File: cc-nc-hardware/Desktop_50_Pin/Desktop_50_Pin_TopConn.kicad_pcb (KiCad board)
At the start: 4 copper layers, 93.7 x 82.6 mm, 112 parts, among them J1 Conn_01x03_Male, J10 Conn_01x03_Male, J11 Conn_01x02_Male, J2 Conn_02x25_Odd_Even, J3 BergFloppy, J4 USB_C_Receptacle, J5 Conn_01x03_Male, J6 SM04B-SRSS-TB(LF)(SN), J7 TERM_BCKF, J8 EPWR, J9 Conn_01x02_Male, Q1 AO3401A, Q2 AO3401A, SW1 SW_MEC_5E, U13 LVT125, U14 LVT125, U15 LVT125, U16 LVT125, U3 AMS1117-2.85, U4 LVT245, U5 LVT245, U6 LVT245, U8 74HC14, U9 LVT245

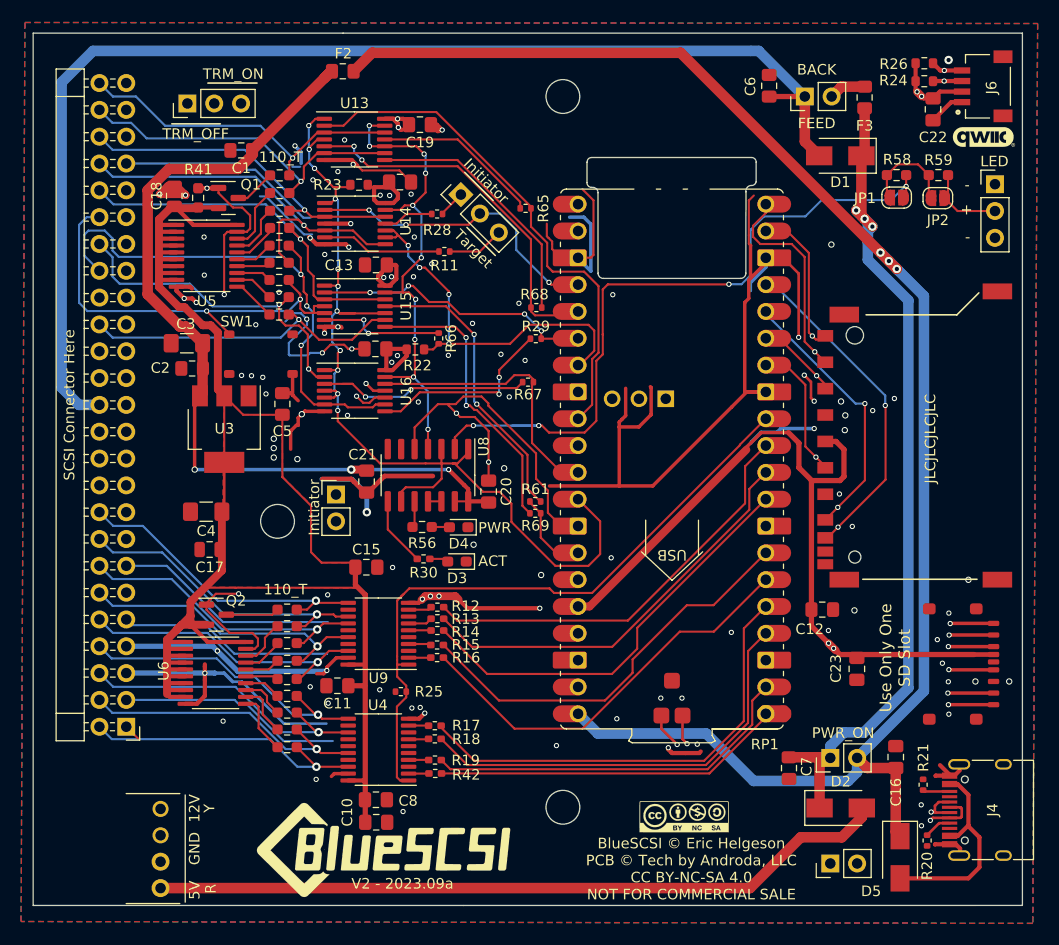
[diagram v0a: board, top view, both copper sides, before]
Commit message: Desktop 2023.10a design
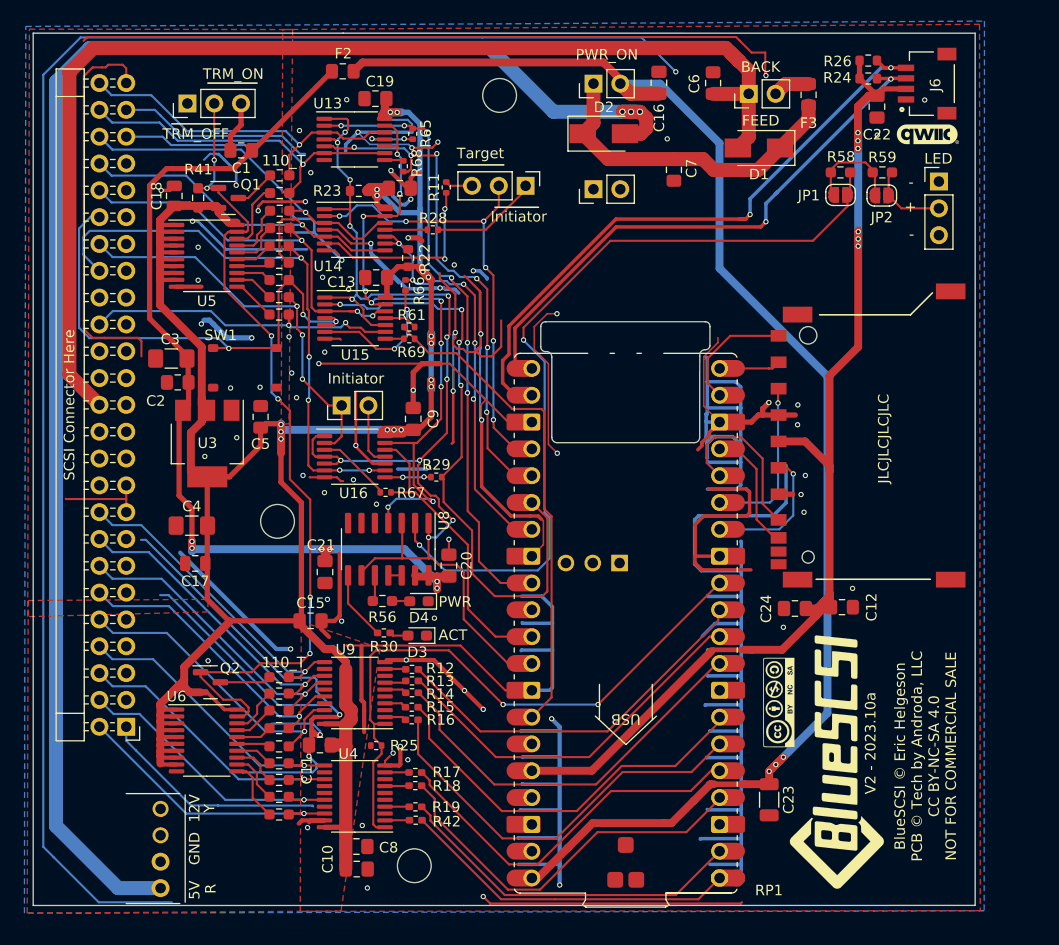
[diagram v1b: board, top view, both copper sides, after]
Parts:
- removed D5: D, Diode_SMD:D_SMA
- removed J4: USB_C_Receptacle, Connector_USB:USB_C_Receptacle_HRO_TYPE-C-31-M-12
- removed R20, R21: 5.1k, Resistor_SMD:R_0402_1005Metric
- removed SD2: MicroSD-TF-06, Library:TF-06_MicroSD
- added C24: 0.1uF, Capacitor_SMD:C_0805_2012Metric_Pad1.18x1.45mm_HandSolder, F.Cu at (172.1, 118.3)
- C23: value 4.7uF -> 20uF; footprint Capacitor_SMD:C_0805_2012Metric_Pad1.18x1.45mm_HandSolder -> Capacitor_SMD:C_1206_3216Metric
- J11: value Conn_01x02_Male -> ACK_En
- moved C16 67.7 mm to (159.3, 68.5)
- moved D2 67.7 mm to (154.0, 73.3)
- moved J8 67.7 mm to (153.1, 68.6)
- moved J9 67.7 mm to (153.1, 78.6)
- moved C7 57.7 mm to (160.7, 76.8)
- moved R61 20.4 mm to (135.6, 91.6)
- moved R69 20.4 mm to (135.6, 92.7)
- moved R68 18.4 mm to (135.1, 76.4), turned to 90 degrees
- moved R67 17.1 mm to (133.4, 107.3)
- moved RP1 16.2 mm to (156.1, 119.8)
- moved R29 16.1 mm to (138.2, 105.8)
- moved H3 15.1 mm to (136.1, 142.6)
- moved C23 14.9 mm to (169.7, 136.4)
- moved G*** 14.0 mm to (170.6, 127.2), turned to 90 degrees
- moved R65 12.8 mm to (135.9, 73.3), turned to 90 degrees
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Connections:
- C23 pad 1: +3V3 -> +5VP
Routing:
- net GND: track 569.8 -> 946.8 mm, vias 100 -> 81
- net Net-(D2-Pad2): track 70.1 -> 151.4 mm, vias 0 -> 3
- net SD_D3_CS: track 58.1 -> 4.21 mm, vias 2 -> 0
- net SD_D1: track 59.6 -> 10.7 mm, vias 3 -> 0
- net +3V3: track 149.2 -> 109.8 mm, vias 4 -> 6
- net SD_D2: track 50.7 -> 11.5 mm, vias 2 -> 0
- net Net-(R61-Pad1): track 7.97 -> 46.5 mm
- net SD_D0_MISO: track 54.6 -> 16.3 mm, vias 3 -> 0
- net Net-(C7-Pad1): track 82.0 -> 45.2 mm, vias 3 -> 0
- net USB_DM: track 35.5 -> 0.00 mm, vias 2 -> 0
- net USB_DP: track 33.0 -> 0.00 mm, vias 2 -> 0
- net oMSG_iBSY: track 25.4 -> 58.0 mm
- net SD_CLK: track 45.1 -> 13.1 mm, vias 2 -> 1
- net SD_CMD_MOSI: track 44.9 -> 16.0 mm, vias 2 -> 1
- net +5F: track 121.4 -> 93.3 mm, vias 3 -> 6
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- removed copper zone on In1.Cu, net GND
- removed copper zone on In2.Cu, net GND
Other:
- board size 93.7 x 82.6 mm -> 89.2 x 82.6 mm
- copper layers 4 -> 2
- board text added: "V2 - 2023.10a"
- board text added: "© 2022 - 2023 Tech by Androda, LLC Licensed Attribution-NonCommercial-ShareAlike 4.0 International (CC BY-NC-SA 4.0) https://creativecommons.org/licenses/by-nc-sa/4.0/legalcode"
- board text removed: "Use Only One SD Slot"
- board text removed: "V2 - 2023.09a"
